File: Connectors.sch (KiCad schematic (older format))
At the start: 17 parts, among them J1 Conn_01x03, J10 Conn_01x03, J11 Conn_01x02, J12 Conn_01x03, J13 Conn_01x02, J14 Conn_01x04, J15 Conn_01x04, J16 Conn_01x01, J17 Conn_01x01, J2 USB_B_Micro, J3 Conn_01x08, J4 Conn_01x08, J5 Conn_01x04, J6 Conn_01x02, J7 Conn_01x02, J8 Conn_01x04, J9 Conn_01x04

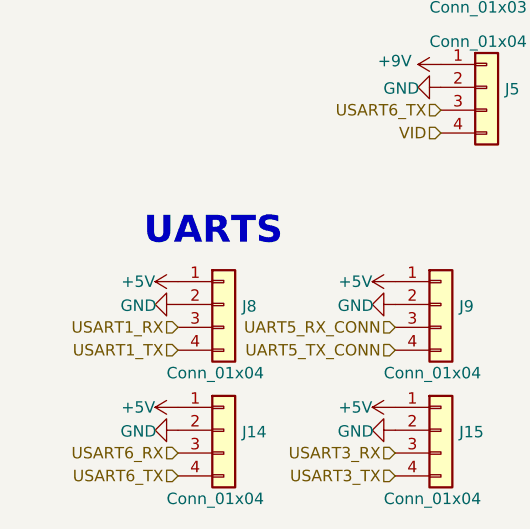
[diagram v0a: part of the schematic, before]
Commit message: Finished routing
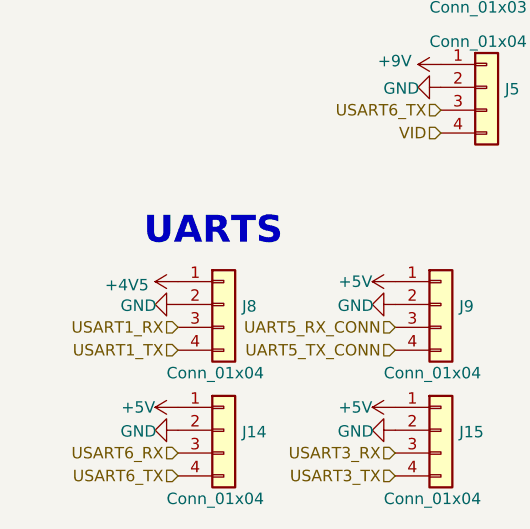
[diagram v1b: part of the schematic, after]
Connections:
- net +5V: no longer J8.1 (Pin_1)
- new net +4V5: J8.1 (Pin_1)
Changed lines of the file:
@@
 	0    1    1    0
 $EndComp
-$Comp
-L power:+5V #PWR?
-U 1 1 60A8659D
-P 1650 6600
-AR Path="/60A8659D" Ref="#PWR?"  Part="1"
-AR Path="/60A7361B/60A8659D" Ref="#PWR080"  Part="1"
-F 0 "#PWR080" H 1650 6450 50  0001 C CNN
-F 1 "+5V" V 1650 6700 50  0000 L CNN
-F 2 "" H 1650 6600 50  0001 C CNN
-F 3 "" H 1650 6600 50  0001 C CNN
-	1    1650 6600
-	0    -1   -1   0
-$EndComp
 Text Notes 1500 6450 0    118  ~ 24
 UARTS
@@
 	1    0    0    -1
 $EndComp
+$Comp
+L power:+4V5 #PWR?
+U 1 1 6186F9D7
+P 1700 6600
+F 0 "#PWR?" H 1875 6675 50  0001 C CNN
+F 1 "+4V5" V 1685 6778 50  0000 L CNN
+F 2 "" H 1700 6600 50  0001 C CNN
+F 3 "" H 1700 6600 50  0001 C CNN
+	1    1700 6600
+	0    -1   -1   0
+$EndComp
 $EndSCHEMATC
